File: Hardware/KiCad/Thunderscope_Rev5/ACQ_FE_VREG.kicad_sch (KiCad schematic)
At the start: 70 parts, among them U13 LM27761, U14 TPS7A9101, U15 TPS7A9101, U16 TPS7A2033, U17 TPS61023, U9 TPS7A2033

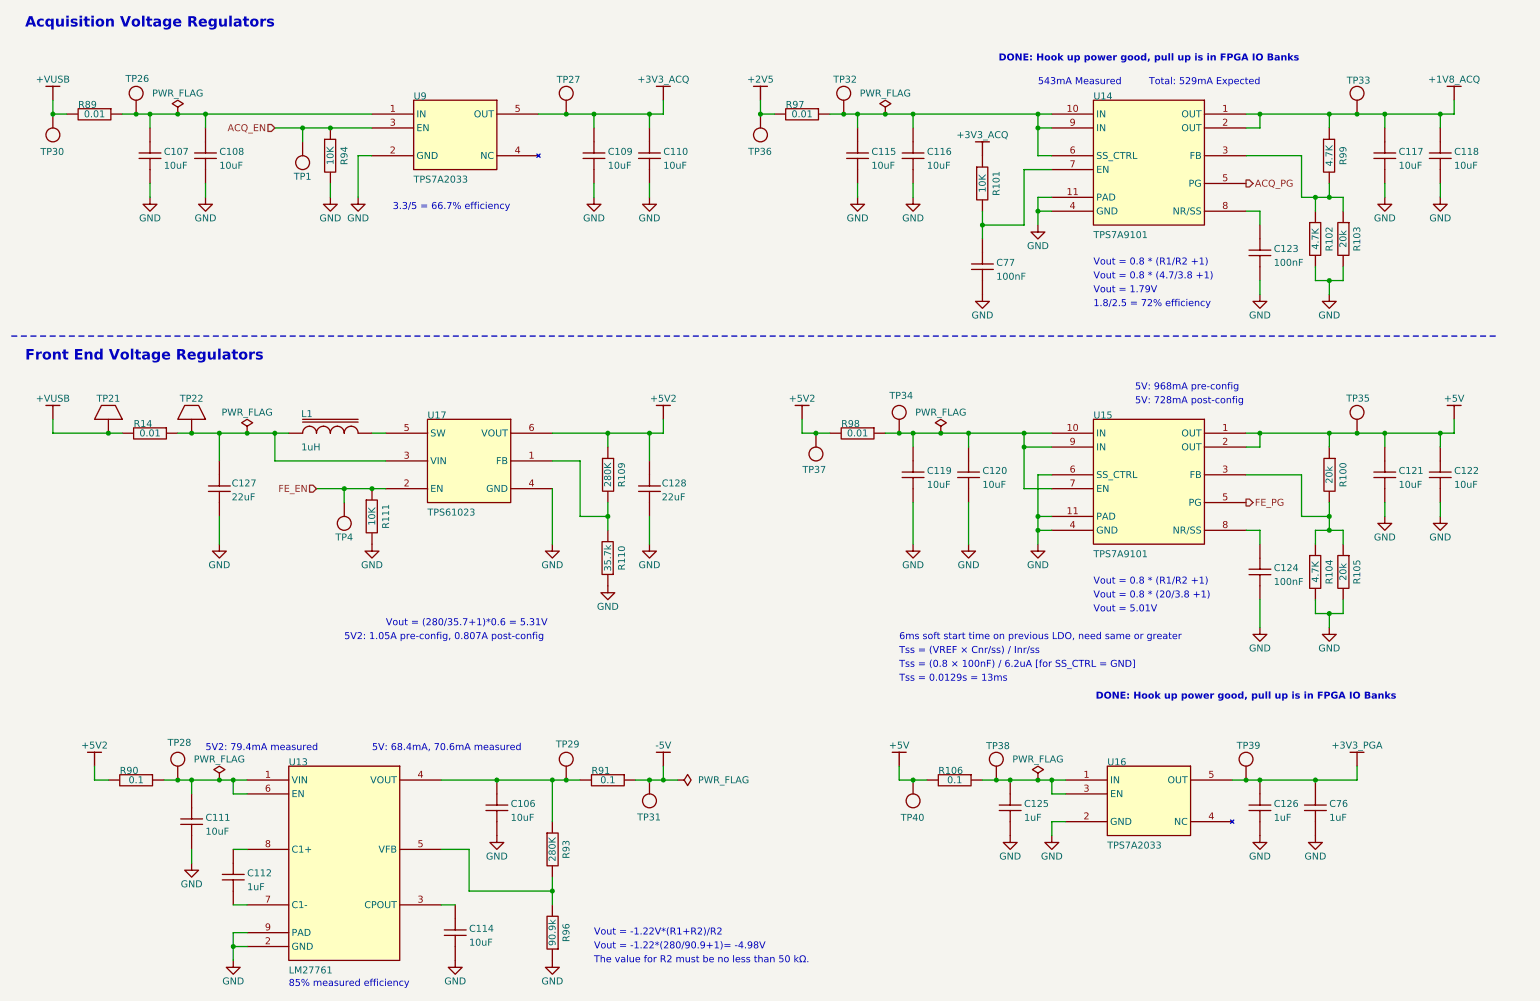
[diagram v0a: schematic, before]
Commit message: Refactored Schematic
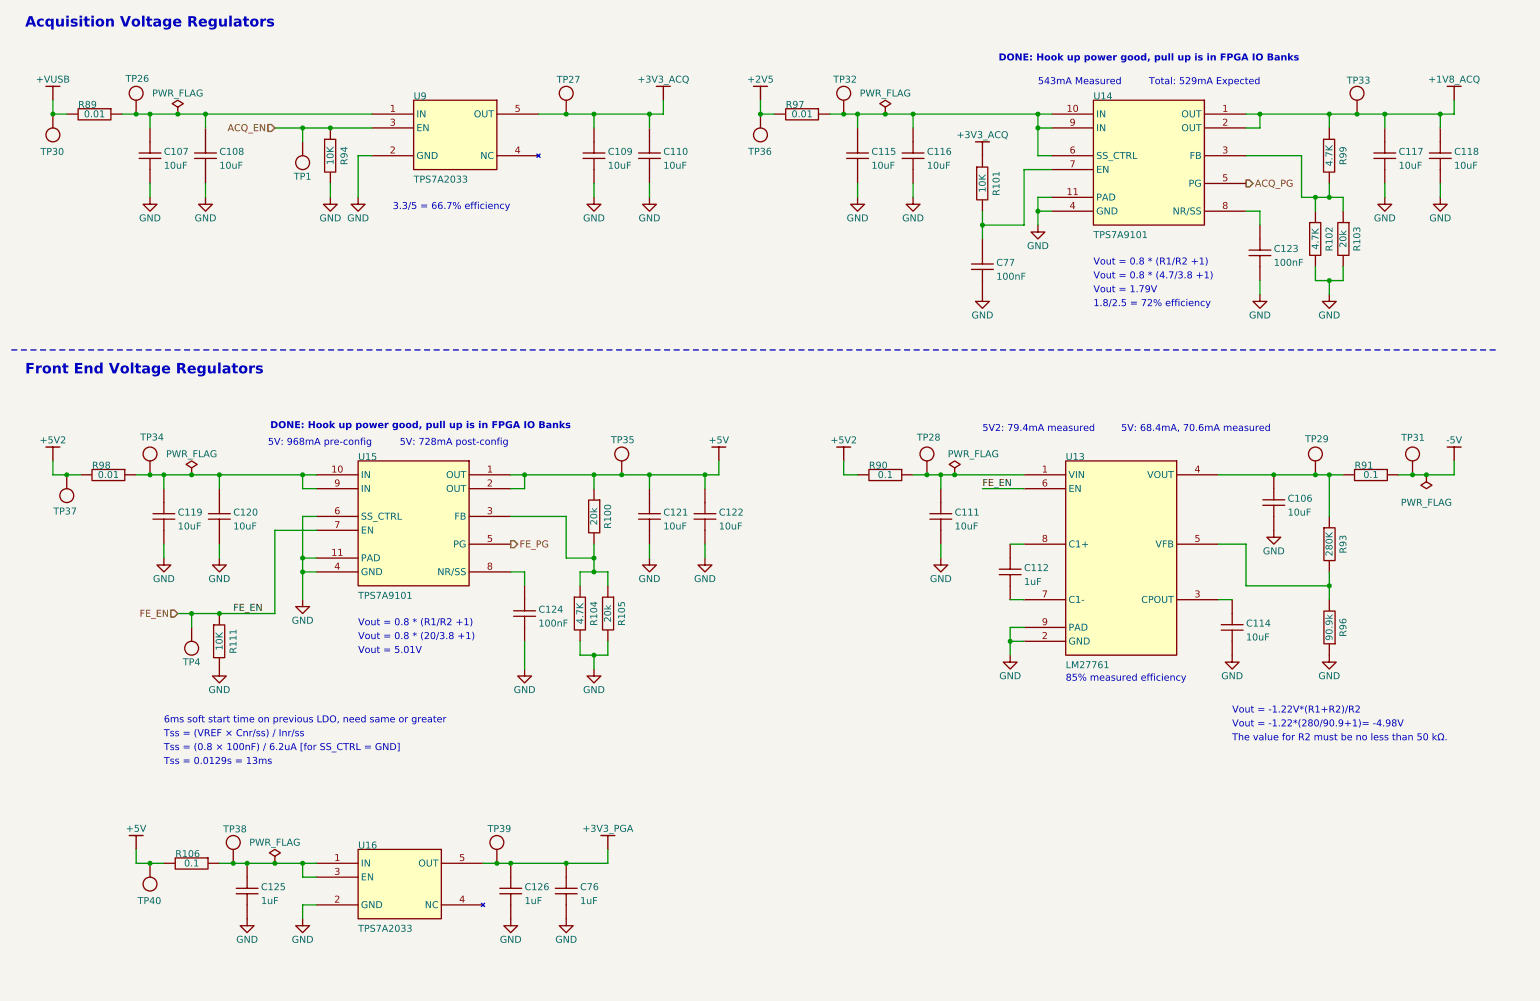
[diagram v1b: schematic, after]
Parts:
- removed C127, C128: 22uF, Thunderscope_Rev5:GEN_C_0805, symbol Thunderscope_Rev5:CAP 22uF 25V X5R 0805
- removed L1: 1uH, Thunderscope_Rev5:GEN_L_1210, symbol Thunderscope_Rev5:IND 1uH 5.5A 32 MOHM 1210
- removed R109: 280K, Thunderscope_Rev5:GEN_R_0402, symbol Thunderscope_Rev5:RES 280K OHM 1% 1/16W 0402
- removed R110: 35.7k, Thunderscope_Rev5:GEN_R_0402, symbol Thunderscope_Rev5:RES 35.7K OHM 1% 1/16W 0402
- removed R14: 0.01, Thunderscope_Rev5:GEN_R_0603, symbol Thunderscope_Rev5:RES 0.01 OHM 1% 1/4W 0603
- removed TP21, TP22: 5015, Thunderscope_Rev5:KEY_5015, symbol Thunderscope_Rev5:TP KEYSTONE 5015
- removed U17: TPS61023, Thunderscope_Rev5:TI_SOT563_DRL0006A, symbol Thunderscope_Rev5:IC BOOST TPS61023
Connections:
- net FE_EN: now also U13.6 (EN), U15.7 (EN)
- net at C119.2, C120.2, R98.2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: no longer U15.7 (EN)
- net at C111.2, R90.2, TP28.1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: no longer U13.6 (EN)
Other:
- note removed: "5V2: 1.05A pre-config, 0.807A post-config"
- note removed: "Vout = (280/35.7+1)*0.6 = 5.31V"
- moved on the sheet: C106, C111, C112, C114, C119, C120, C121, C122, C124, C125, C126, C76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

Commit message: Rev 5 WIP
Added probe comp variants
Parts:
- C106, C107, C108, C109, C110, C111, C114, C115, C116, C117, C118, C119, C120, C121, C122: symbol Thunderscope_Rev5:CAP 10uF 10V X5R 0603 -> Thunderscope_Rev5:CAP 10uF 25V X5R 0603; HOUSE PART NUMBER C-10uF-0603-002 -> (none); MANUFACTURER PART NUMBER GRM188R61A106ME69D -> GRM188R61E106MA73D; SUPPLIER PART NUMBER 1 81-GRM188R61A106ME9D -> 81-GRM188R61E106MA3D; VOLTAGE RATING 10V -> 25V
- U14, U15: MANUFACTURER PART NUMBER TPS7A9101DSKT -> TPS7A9101DSKR; SUPPLIER 1 Digi-Key -> Texas Instruments; SUPPLIER PART NUMBER 1 296-45298-1-ND -> TPS7A9101DSKR
